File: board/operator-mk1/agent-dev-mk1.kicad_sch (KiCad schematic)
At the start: 7 parts, among them J1 Slide Switch, J2 Microphone, J3 Buttons, J4 Speaker, J8 TRRS Socket, M1 XIAO ESP32

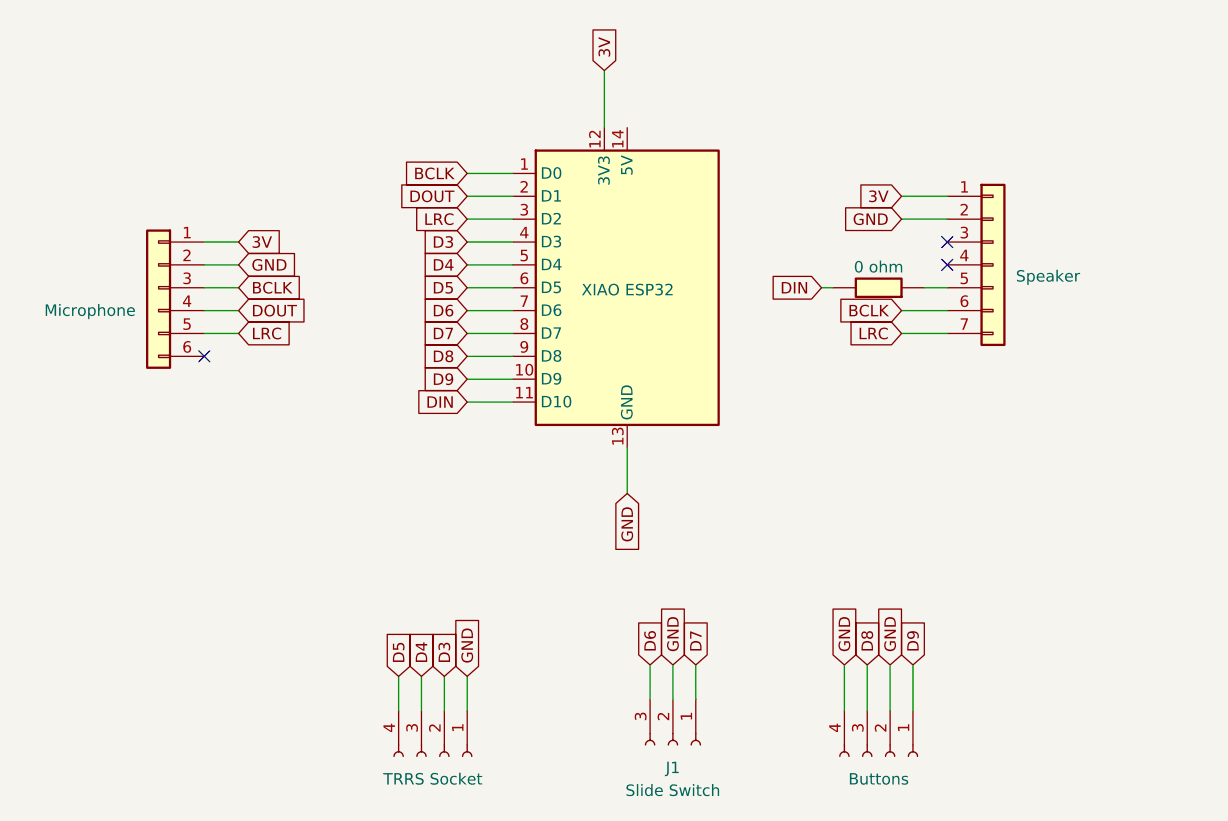
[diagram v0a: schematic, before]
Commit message: archive
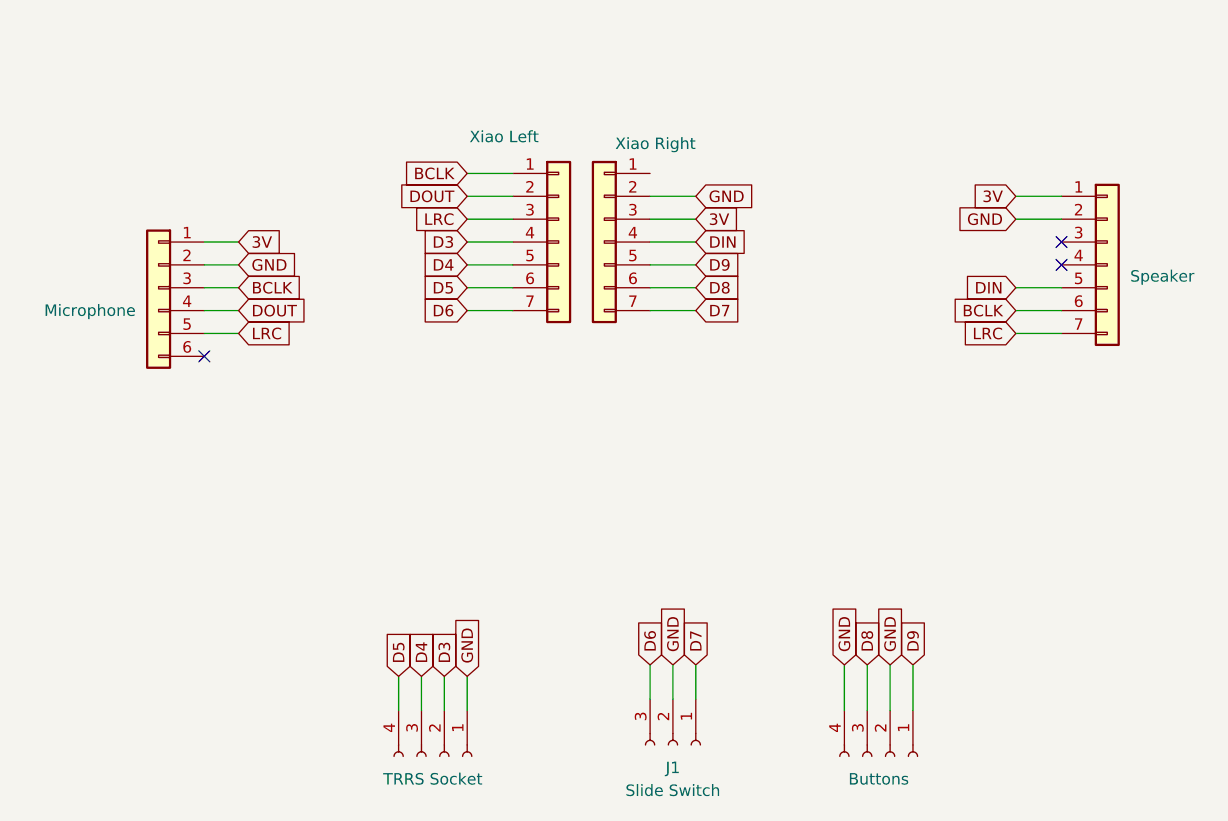
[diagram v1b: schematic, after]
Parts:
- removed M1: XIAO ESP32, fab:Module_XIAO_Generic_SocketSMD, symbol fab:Module_XIAO_Generic_SocketSMD
- removed R1: 0 ohm, fab:R_1206, symbol fab:R_1206
- added J5: Xiao Left, Connector_PinSocket_2.54mm:PinSocket_1x07_P2.54mm_Vertical, symbol Connector_Generic:Conn_01x07
- added J6: Xiao Right, Connector_PinSocket_2.54mm:PinSocket_1x07_P2.54mm_Vertical, symbol Connector_Generic:Conn_01x07
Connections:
- net 3V: now also J6.3 (Pin_3)
- net BCLK: now also J5.1 (Pin_1)
- net D3: now also J5.4 (Pin_4)
- net D4: now also J5.5 (Pin_5)
- net D5: now also J5.6 (Pin_6)
- net D6: now also J5.7 (Pin_7)
- net D7: now also J6.7 (Pin_7)
- net D8: now also J6.6 (Pin_6)
- net D9: now also J6.5 (Pin_5)
- net DIN: now also J4.5 (Pin_5), J6.4 (Pin_4)
- net DOUT: now also J5.2 (Pin_2)
- net GND: now also J6.2 (Pin_2)
- net LRC: now also J5.3 (Pin_3)
